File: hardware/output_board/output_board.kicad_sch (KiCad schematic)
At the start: 2 parts, among them J1 I/O, J2 conn_2x2

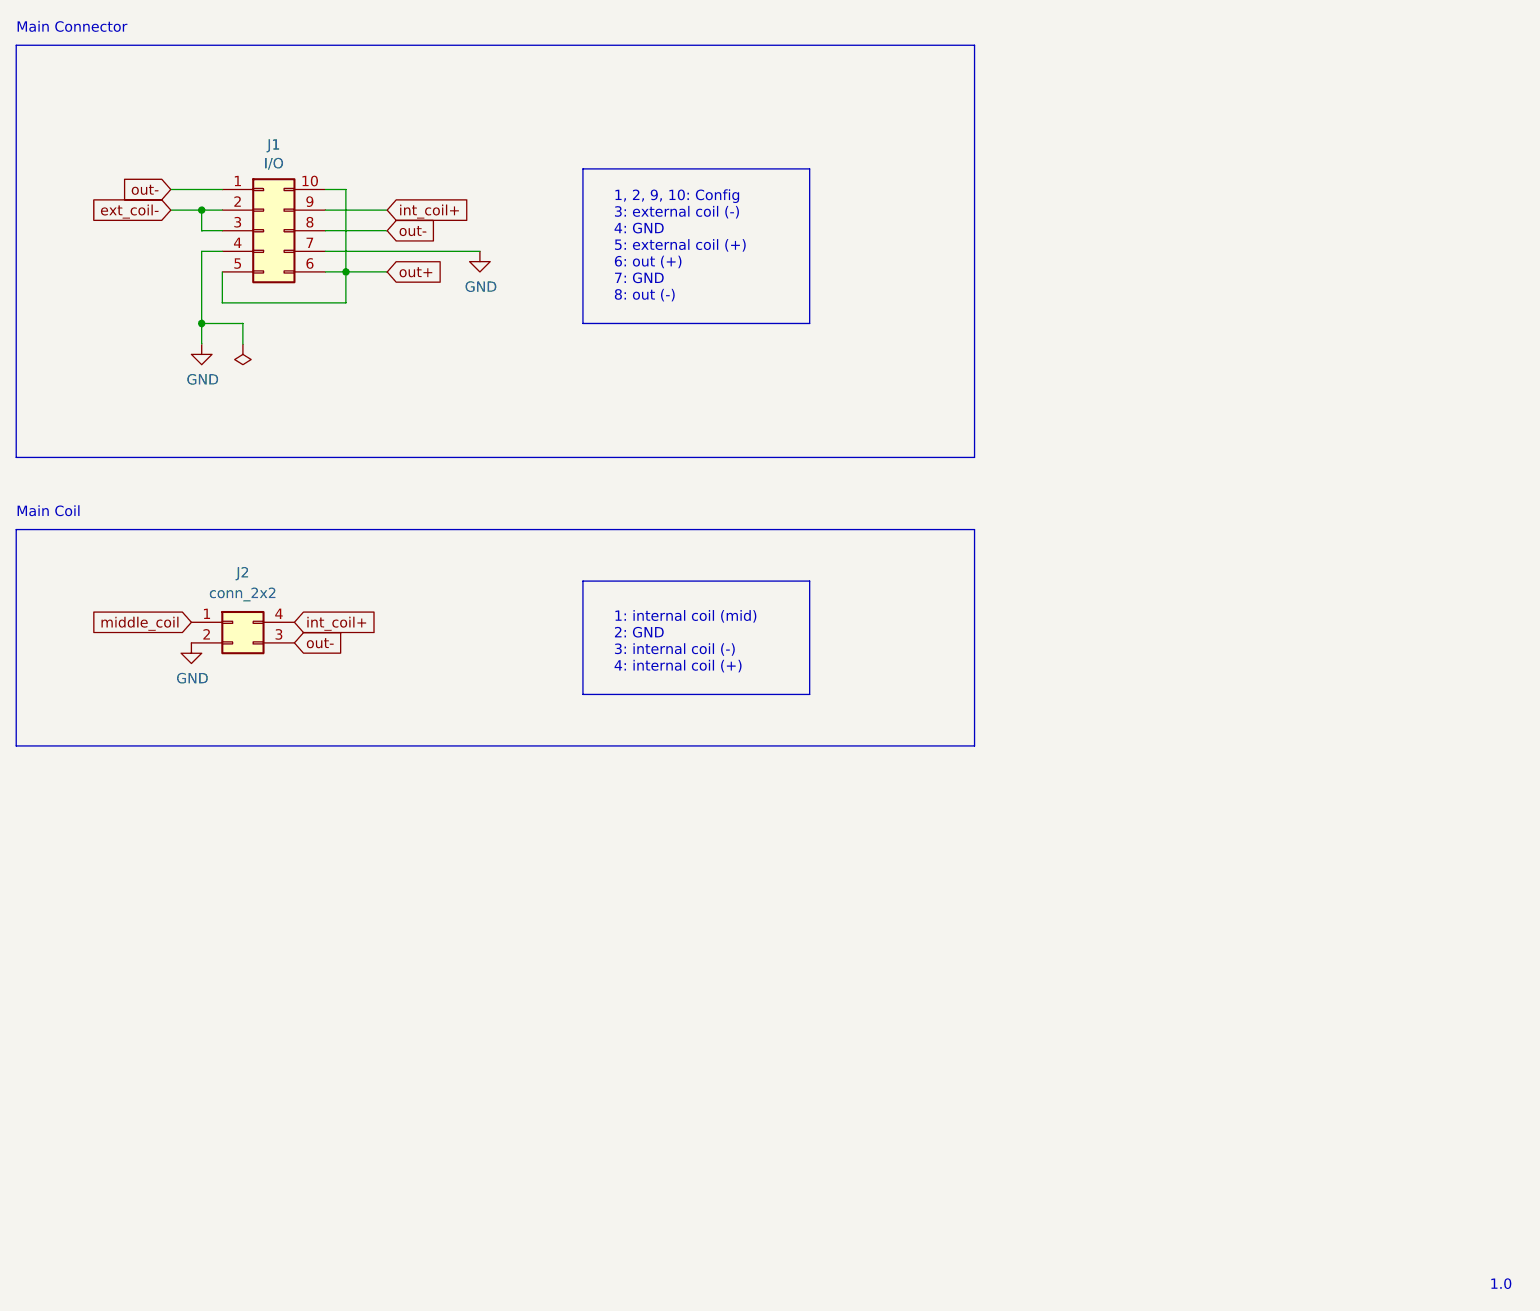
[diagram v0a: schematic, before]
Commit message: Output board and base board review
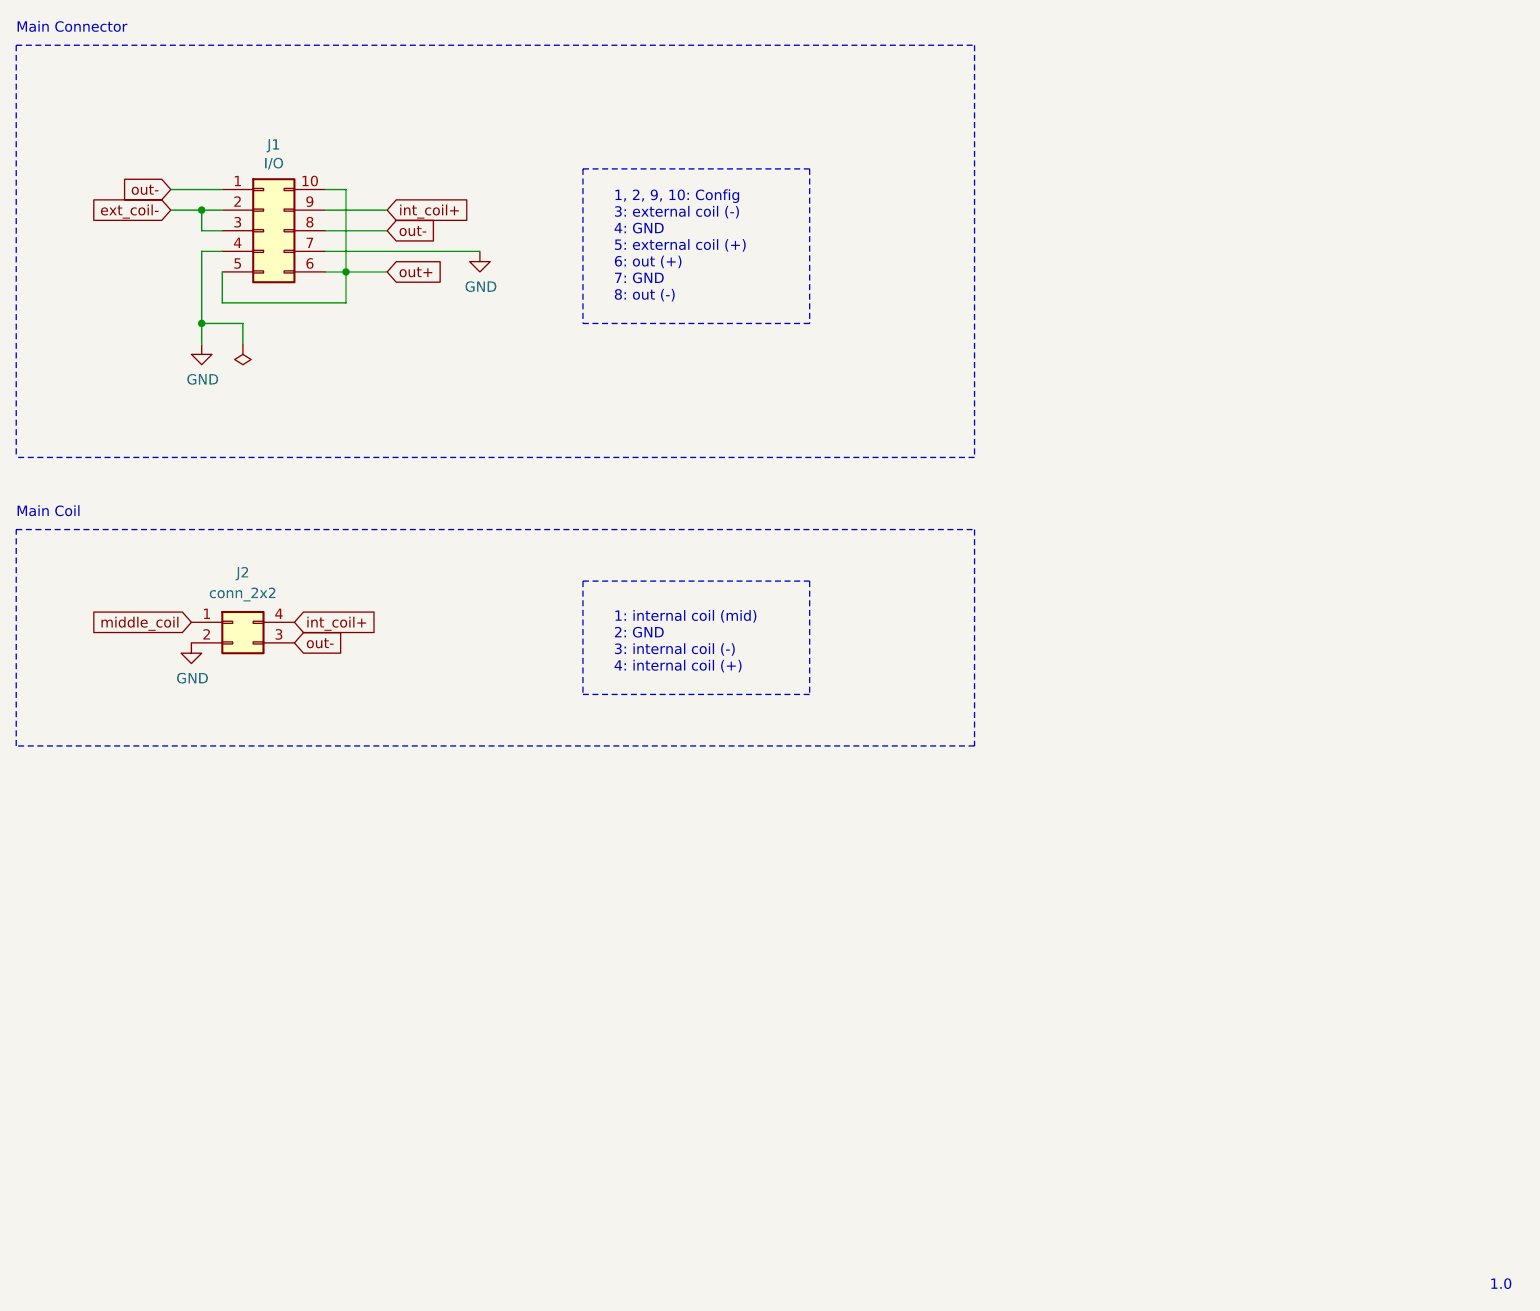
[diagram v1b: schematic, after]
